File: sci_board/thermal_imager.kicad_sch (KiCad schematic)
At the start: 0 parts

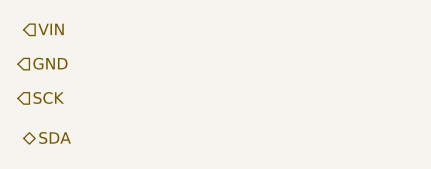
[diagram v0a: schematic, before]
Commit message: start SCI pcb
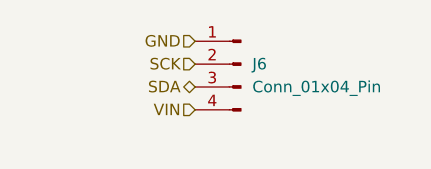
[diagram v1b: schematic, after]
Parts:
- added J6: Conn_01x04_Pin, Connector_PinHeader_2.54mm:PinHeader_1x04_P2.54mm_Vertical, symbol Connector:Conn_01x04_Pin
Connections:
- net GND: now also J6.1 (Pin_1)
- net SCK: now also J6.2 (Pin_2)
- net SDA: now also J6.3 (Pin_3)
- net VIN: now also J6.4 (Pin_4)
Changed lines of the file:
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@@
 	(hierarchical_label "SCK"
 		(shape input)
-		(at 28.575 35.56 0)
+		(at 48.26 31.75 180)
 		(fields_autoplaced yes)
 		(effects
@@
 				(size 1.27 1.27)
 			)
-			(justify left)
+			(justify right)
 		)
 	)
 	(hierarchical_label "SDA"
 		(shape bidirectional)
-		(at 29.21 40.005 0)
+		(at 48.26 34.29 180)
 		(fields_autoplaced yes)
 		(effects
@@
 				(size 1.27 1.27)
 			)
-			(justify left)
+			(justify right)
 		)
 	)
 	(hierarchical_label "GND"
 		(shape input)
-		(at 28.575 31.75 0)
+		(at 48.26 29.21 180)
 		(fields_autoplaced yes)
 		(effects
@@
 				(size 1.27 1.27)
 			)
-			(justify left)
+			(justify right)
 		)
 	)
 	(hierarchical_label "VIN"
 		(shape input)
-		(at 29.21 27.94 0)
+		(at 48.26 36.83 180)
 		(fields_autoplaced yes)
 		(effects
@@
 				(size 1.27 1.27)
 			)
-			(justify left)
+			(justify right)
 		)
 	)
+	(symbol
+		(lib_id "Connector:Conn_01x04_Pin")
+		(at 53.34 31.75 0)
+		(mirror y)
+		(unit 1)
+		(exclude_from_sim no)
+		(in_bom yes)
+		(on_board yes)
+		(dnp no)
+		(fields_autoplaced yes)
+		(property "Reference" "J6"
+			(at 54.61 31.7499 0)
+			(effects
+				(font
+					(size 1.27 1.27)
+				)
+				(justify right)
+			)
+		)
+		(property "Value" "Conn_01x04_Pin"
+			(at 54.61 34.2899 0)
+			(effects
+				(font
+					(size 1.27 1.27)
+				)
+				(justify right)
+			)
+		)
+		(property "Footprint" "Connector_PinHeader_2.54mm:PinHeader_1x04_P2.54mm_Vertical"
+			(at 53.34 31.75 0)
+			(effects
+				(font
+					(size 1.27 1.27)
+				)
+				(hide yes)
+			)
+		)
+		(property "Datasheet" "~"
+			(at 53.34 31.75 0)
+			(effects
+				(font
+					(size 1.27 1.27)
+				)
+				(hide yes)
+			)
+		)
+		(property "Description" "Generic connector, single row, 01x04, script generated"
+			(at 53.34 31.75 0)
+			(effects
+				(font
+					(size 1.27 1.27)
+				)
+				(hide yes)
+			)
+		)
+		(pin "2"
+		)
+		(pin "1"
+		)
+		(pin "3"
+		)
+		(pin "4"
+		)
+		(instances
+			(project ""
+				(path "/b4b2c88d-f6cd-4e60-862d-e21f68728580/b65d9c5b-bcd6-4ca1-83d4-ac547dcb4ba6"
+					(reference "J6")
+					(unit 1)
+				)
+			)
+		)
+	)
